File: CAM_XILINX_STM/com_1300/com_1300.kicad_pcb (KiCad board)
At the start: 4 copper layers, 50 x 75.9 mm, 112 parts, among them J1 MEC1-108-01-S-D-RA1-SL, J2 9-68RD-0.635SF, U1 LT1963AxST-3.3, U2 LP3982IMM-ADJ, U3 LTC3411EMS, U5 STM32F415RGTx, U6 AM29LV320DT90EC, U7 TC74LCX373FT, Y1 40mHZ, Y2 16mHz

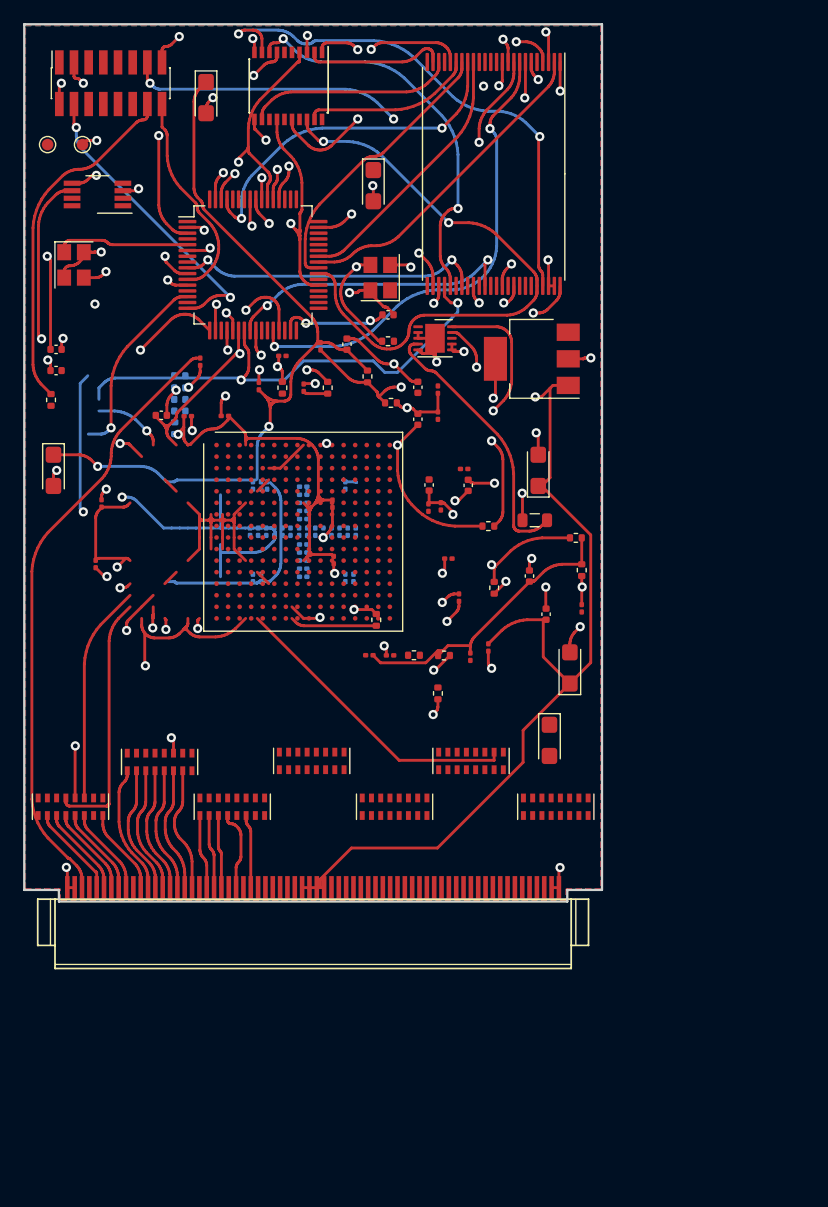
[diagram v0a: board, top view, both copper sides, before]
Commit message: 2342342
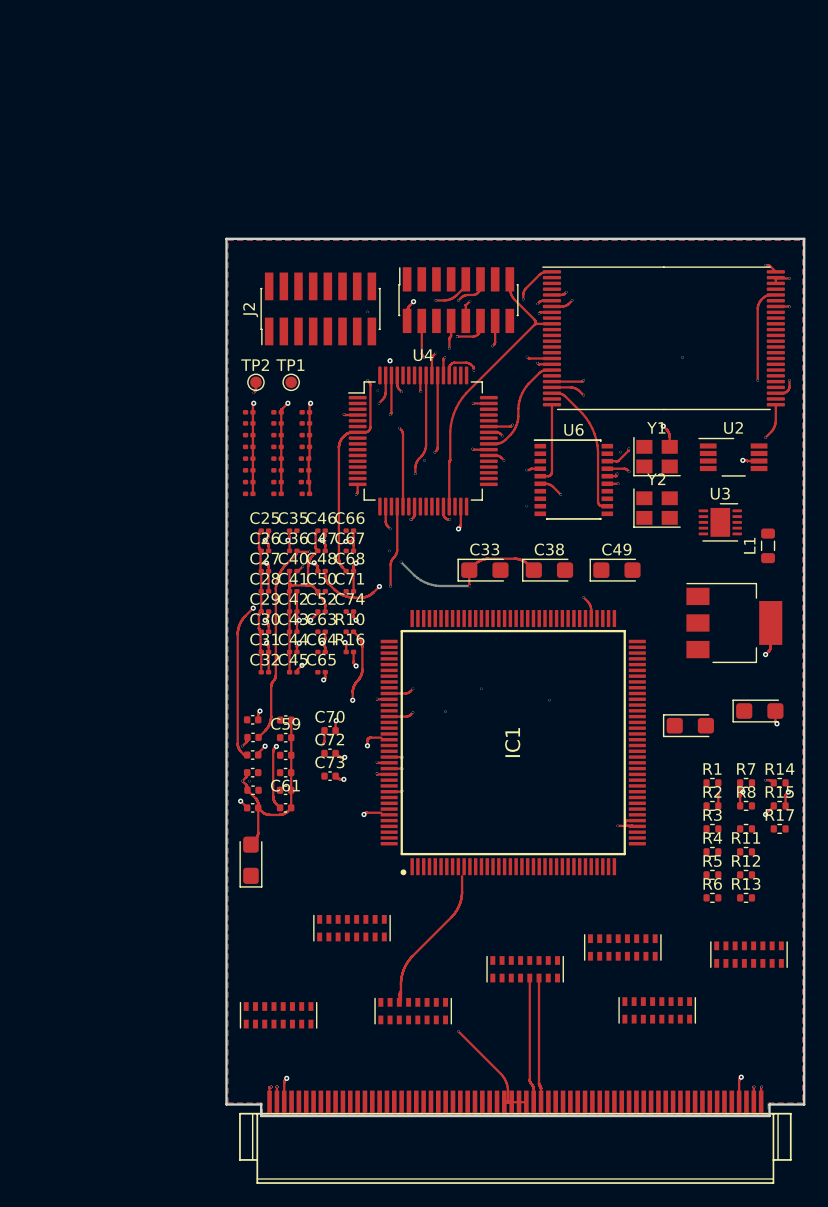
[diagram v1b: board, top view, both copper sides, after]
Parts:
- removed the C24 at (32.4, 39.0)
- removed the C24 at (50.8, 36.7)
- removed the C24 at (50.8, 39.0)
- removed the C24 at (63.2, 55.6)
- removed the C24 at (21.2, 51.8)
- removed the C24 at (17.8, 33.2)
- removed the C24 at (41.7, 46.6)
- removed the C24 at (49.1, 39.3)
- removed the C24 at (21.7, 46.5)
- removed the C24 at (53.6, 59.8)
- removed the C24 at (51.1, 46.8)
- removed the C24 at (50.0, 46.9)
- removed the C24 at (49.1, 36.5)
- removed the C24 at (41.8, 51.4)
- removed the C24 at (17.8, 35.1)
- removed the C24 at (39.1, 46.5)
- removed the C24 at (39.1, 45.8)
- removed the C24 at (36.0, 45.0)
- removed the C24 at (28.5, 37.5)
- removed the C24 at (43.5, 53.0)
- removed the C24 at (39.1, 45.1)
- removed the C24 at (40.2, 49.0)
- removed the C24 at (46.5, 30.2)
- removed the C24 at (43.7, 49.0)
- removed the C24 at (39.1, 47.2)
- removed the C24 at (39.1, 50.8)
- removed the C24 at (43.0, 49.0)
- removed the C24 at (35.2, 49.0)
- removed the C24 at (42.3, 49.0)
- removed the C24 at (35.5, 53.0)
- removed the C24 at (39.1, 52.2)
- removed the C24 at (38.0, 49.0)
- removed the C24 at (34.5, 49.0)
- removed the C24 at (53.4, 45.0)
- removed the C24 at (34.8, 45.0)
- removed the C24 at (39.1, 47.9)
- removed the C24 at (39.1, 52.9)
- removed the C24 at (39.5, 49.0)
- removed the C24 at (40.9, 49.0)
- removed the C24 at (39.1, 51.5)
- removed the C24 at (36.6, 49.0)
- removed the C24 at (42.8, 45.0)
- removed the C24 at (41.6, 49.0)
- removed the C24 at (37.3, 49.0)
- removed the C24 at (29.2, 39.0)
- removed the C24 at (35.9, 49.0)
- removed the C24 at (42.8, 53.0)
- removed the C24 at (34.8, 53.0)
- removed the C24 at (35.5, 45.0)
- removed the C24 at (39.1, 50.1)
- removed the C24 at (38.8, 49.0)
- removed the C24 at (51.7, 51.3)
- removed the C24 at (44.9, 59.7)
- removed the C24 at (53.1, 43.6)
- removed the C24 at (37.3, 33.8)
- removed C39: 10uF, Capacitor_Tantalum_SMD:CP_EIA-3216-18_Kemet-A
- removed C62: C-OPEN, Capacitor_SMD:C_0402_1005Metric
- removed R9: 56, Resistor_SMD:R_0402_1005Metric
- removed U: XC3S400-4FT256C, Package_BGA:Xilinx_FTG256
- removed U7: TC74LCX373FT, Package_SO:SSOP-20_4.4x6.5mm_P0.65mm
- added C24: C-OPEN, Capacitor_SMD:C_0402_1005Metric, F.Cu at (41.5, 66.2)
- added C24: C-OPEN, Capacitor_SMD:C_0201_0603Metric, F.Cu at (38.3, 61.2)
- added C24: C-OPEN, Capacitor_SMD:C_0201_0603Metric, F.Cu at (35.8, 52.4)
- added C24: C-OPEN, Capacitor_SMD:C_0201_0603Metric, F.Cu at (38.3, 54.2)
- added C24: C-OPEN, Capacitor_SMD:C_0201_0603Metric, F.Cu at (39.4, 45.7)
- added C24: C-OPEN, Capacitor_SMD:C_0201_0603Metric, F.Cu at (40.7, 61.2)
- added C24: C-OPEN, Capacitor_SMD:C_0201_0603Metric, F.Cu at (35.8, 57.7)
- added C24: C-OPEN, Capacitor_SMD:C_0402_1005Metric, F.Cu at (37.6, 71.4)
- added C24: C-OPEN, Capacitor_SMD:C_0201_0603Metric, F.Cu at (36.9, 38.7)
- added C24: C-OPEN, Capacitor_SMD:C_0201_0603Metric, F.Cu at (38.3, 52.4)
- added C24: C-OPEN, Capacitor_SMD:C_0201_0603Metric, F.Cu at (35.8, 61.2)
- added C24: C-OPEN, Capacitor_SMD:C_0201_0603Metric, F.Cu at (34.5, 38.7)
- added C24: C-OPEN, Capacitor_SMD:C_0201_0603Metric, F.Cu at (40.7, 50.7)
- added C24: C-OPEN, Capacitor_SMD:C_0201_0603Metric, F.Cu at (43.2, 55.9)
- added C24: C-OPEN, Capacitor_SMD:C_0201_0603Metric, F.Cu at (36.9, 43.7)
- added C24: C-OPEN, Capacitor_SMD:C_0201_0603Metric, F.Cu at (34.5, 40.6)
- added C24: C-OPEN, Capacitor_SMD:C_0201_0603Metric, F.Cu at (36.9, 41.7)
- added C24: C-OPEN, Capacitor_SMD:C_0201_0603Metric, F.Cu at (40.7, 57.7)
- added C24: C-OPEN, Capacitor_SMD:C_0201_0603Metric, F.Cu at (38.3, 57.7)
- added C24: C-OPEN, Capacitor_SMD:C_0201_0603Metric, F.Cu at (38.3, 59.4)
- added C24: C-OPEN, Capacitor_SMD:C_0201_0603Metric, F.Cu at (34.5, 39.6)
- added C24: C-OPEN, Capacitor_SMD:C_0201_0603Metric, F.Cu at (36.9, 42.7)
- added C24: C-OPEN, Capacitor_SMD:C_0201_0603Metric, F.Cu at (34.5, 43.7)
- added C24: C-OPEN, Capacitor_SMD:C_0402_1005Metric, F.Cu at (34.8, 68.3)
- added C24: C-OPEN, Capacitor_SMD:C_0201_0603Metric, F.Cu at (39.3, 42.7)
- added C24: C-OPEN, Capacitor_SMD:C_0201_0603Metric, F.Cu at (35.8, 55.9)
- added C24: C-OPEN, Capacitor_SMD:C_0201_0603Metric, F.Cu at (35.8, 54.2)
- added C24: C-OPEN, Capacitor_SMD:C_0201_0603Metric, F.Cu at (34.5, 41.7)
- added C24: C-OPEN, Capacitor_SMD:C_0201_0603Metric, F.Cu at (36.9, 39.6)
- added C24: C-OPEN, Capacitor_SMD:C_0201_0603Metric, F.Cu at (39.3, 43.7)
- added C24: C-OPEN, Capacitor_SMD:C_0201_0603Metric, F.Cu at (35.8, 59.4)
- added C24: C-OPEN, Capacitor_SMD:C_0201_0603Metric, F.Cu at (36.9, 44.7)
- added C24: C-OPEN, Capacitor_SMD:C_0201_0603Metric, F.Cu at (34.5, 42.7)
- added C24: C-OPEN, Capacitor_SMD:C_0201_0603Metric, F.Cu at (35.8, 50.7)
- added C24: C-OPEN, Capacitor_SMD:C_0402_1005Metric, F.Cu at (37.6, 72.9)
- added C24: C-OPEN, Capacitor_SMD:C_0201_0603Metric, F.Cu at (34.5, 44.7)
- added C24: C-OPEN, Capacitor_SMD:C_0201_0603Metric, F.Cu at (43.2, 54.2)
- added C24: C-OPEN, Capacitor_SMD:C_0201_0603Metric, F.Cu at (43.2, 52.4)
- added C24: C-OPEN, Capacitor_SMD:C_0201_0603Metric, F.Cu at (36.9, 45.7)
- added C24: C-OPEN, Capacitor_SMD:C_0201_0603Metric, F.Cu at (40.7, 48.9)
- added C24: C-OPEN, Capacitor_SMD:C_0402_1005Metric, F.Cu at (41.5, 68.2)
- added C24: C-OPEN, Capacitor_SMD:C_0201_0603Metric, F.Cu at (36.9, 40.6)
- added C24: C-OPEN, Capacitor_SMD:C_0402_1005Metric, F.Cu at (34.8, 65.3)
- added C24: C-OPEN, Capacitor_SMD:C_0201_0603Metric, F.Cu at (39.4, 38.7)
- added C24: C-OPEN, Capacitor_SMD:C_0201_0603Metric, F.Cu at (35.8, 48.9)
- added C24: C-OPEN, Capacitor_SMD:C_0201_0603Metric, F.Cu at (40.7, 59.4)
- added C24: C-OPEN, Capacitor_SMD:C_0201_0603Metric, F.Cu at (39.4, 41.7)
- added C24: C-OPEN, Capacitor_SMD:C_0201_0603Metric, F.Cu at (34.5, 45.7)
- added C24: C-OPEN, Capacitor_SMD:C_0201_0603Metric, F.Cu at (43.2, 50.7)
- added C24: C-OPEN, Capacitor_SMD:C_0201_0603Metric, F.Cu at (39.3, 44.7)
- added C24: C-OPEN, Capacitor_SMD:C_0201_0603Metric, F.Cu at (43.2, 48.9)
- added C24: C-OPEN, Capacitor_SMD:C_0201_0603Metric, F.Cu at (38.3, 55.9)
- added C24: C-OPEN, Capacitor_SMD:C_0201_0603Metric, F.Cu at (39.4, 39.6)
- added C24: C-OPEN, Capacitor_SMD:C_0402_1005Metric, F.Cu at (41.5, 70.2)
- added C24: C-OPEN, Capacitor_SMD:C_0201_0603Metric, F.Cu at (39.4, 40.6)
- added C38: 10uF, Capacitor_Tantalum_SMD:CP_EIA-3216-18_Kemet-A, F.Cu at (60.5, 52.3)
- added C48: 100nF, Capacitor_SMD:C_0201_0603Metric, F.Cu at (40.7, 52.4)
- added IC1: XC3S400-4TQ144C, SUNfWGlsaW54X1hDM1MyMDAtNFRRRzE0NEMuemlw:QFP50P2200X2200X160-144N, F.Cu at (57.3, 67.2)
- added J2: Conn_02x10_Top_Bottom, Connector_PinHeader_1.27mm:PinHeader_2x08_P1.27mm_Vertical_SMD, F.Cu at (40.6, 29.7)
- added R8: R-OPEN, Resistor_SMD:R_0402_1005Metric, F.Cu at (77.5, 72.7)
- added U4: STM32F415RGTx, Package_QFP:LQFP-64_10x10mm_P0.5mm, F.Cu at (49.5, 41.1)
- C49: value C-OPEN -> 10uF; footprint Capacitor_SMD:C_0402_1005Metric -> Capacitor_Tantalum_SMD:CP_EIA-3216-18_Kemet-A
- C50: value C-OPEN -> 22pF; footprint Capacitor_SMD:C_0402_1005Metric -> Capacitor_SMD:C_0201_0603Metric; moved to F.Cu
- C51: value C-OPEN -> 10uF; footprint Capacitor_SMD:C_0402_1005Metric -> Capacitor_Tantalum_SMD:CP_EIA-3216-18_Kemet-A; moved to F.Cu
- C53: value 10uF -> 4.7uF; footprint Capacitor_Tantalum_SMD:CP_EIA-3216-18_Kemet-A -> Capacitor_SMD:C_0402_1005Metric
- C54: value 22pF -> 10uF; footprint Capacitor_SMD:C_0201_0603Metric -> Capacitor_Tantalum_SMD:CP_EIA-3216-18_Kemet-A
- C56: value 100nF -> 4.7uF; footprint Capacitor_SMD:C_0201_0603Metric -> Capacitor_SMD:C_0402_1005Metric
- C57, C60: value 4.7uF -> C-OPEN
- C58, C59: value 10uF -> C-OPEN; footprint Capacitor_Tantalum_SMD:CP_EIA-3216-18_Kemet-A -> Capacitor_SMD:C_0402_1005Metric
- C61, R22: moved to F.Cu
- R10: value 100K -> 0; footprint Resistor_SMD:R_0402_1005Metric -> Resistor_SMD:R_0201_0603Metric
- R11: value 100K -> 4.7K
- R12: value R-OPEN -> 330
- R13: value 0 -> 56; footprint Resistor_SMD:R_0201_0603Metric -> Resistor_SMD:R_0402_1005Metric
- R4: value 330 -> 100K
- R5: value 4.7K -> 49.9K
- R7: value 49.9K -> 100K
- U5: value STM32F415RGTx -> AM29LV320DT90EC; footprint Package_QFP:LQFP-64_10x10mm_P0.5mm -> Package_SO:TSOP-I-48_18.4x12mm_P0.5mm
- U6: value AM29LV320DT90EC -> TC74LCX373FT; footprint Package_SO:TSOP-I-48_18.4x12mm_P0.5mm -> Package_SO:SSOP-20_4.4x6.5mm_P0.65mm
- moved R14 71.2 mm to (80.4, 70.7), turned to 0 degrees
- moved R22 60.4 mm to (77.5, 74.7), turned to 0 degrees
- moved U2 59.6 mm to (76.4, 42.6), turned to 0 degrees
- moved Y2 54.7 mm to (69.8, 47.0), turned to 0 degrees
- moved C58 54.3 mm to (37.6, 65.3), turned to 180 degrees
- moved R3 53.3 mm to (74.6, 74.7), turned to 0 degrees
- moved C53 51.9 mm to (34.8, 69.8), turned to 0 degrees
- moved R6 51.1 mm to (74.6, 80.7), turned to 0 degrees
- moved C54 49.4 mm to (78.7, 64.5), turned to 0 degrees
- moved R2 49.0 mm to (74.6, 72.7), turned to 0 degrees
- moved R7 48.1 mm to (77.5, 70.7), turned to 0 degrees
- moved R1 47.7 mm to (74.6, 70.7), turned to 0 degrees
- moved C49 41.6 mm to (66.3, 52.3), turned to 0 degrees
- moved C51 41.3 mm to (34.6, 77.4), turned to 90 degrees
- moved R13 37.3 mm to (77.5, 80.7), turned to 0 degrees
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- renumbered J2 to J3
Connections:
- C49 pad 1: GND -> +3V3
- C49 pad 2: uC_CNTRL1 -> GND
- C50 pad 1: GND -> +1V2
- C50 pad 2: uC_CNTRL4 -> Net-(U3-VFB)
- C51 pad 1: GND -> +3V3
- C51 pad 2: uC_CNTRL2 -> GND
- C52 pad 2: Net-(U2-CC) -> +1V2
- C53 pad 1: +3V3 -> GND
- C53 pad 2: GND -> +2V5
- C54 pad 2: Net-(U3-VFB) -> GND
- C55 pad 1: +3V3 -> +1V2
- C57 pad 1: GND -> /FPGA_CLK1
- C57 pad 2: +2V5 -> GND
- C58 pad 1: +1V2 -> GND
- C58 pad 2: GND -> uC_CNTRL1
- C59 pad 1: +1V2 -> 40MHz_OSC
- C60 pad 2: +1V2 -> uC_CNTRL2
- C61 pad 1: /FPGA_CLK1 -> GND
- C61 pad 2: GND -> uC_CNTRL4
- R10 pad 1: Net-(U2-SET) -> Net-(IC1-IO_L32P_4/GCLK0)
- R10 pad 2: +2V5 -> /FPGA_CLK1
- R11 pad 1: GND -> +3V3
- R11 pad 2: Net-(U2-SET) -> Net-(IC1-IO_L31N_4/INIT_B)
- R12 pad 1: GND -> +2V5
- R12 pad 2: +2V5 -> FPGA_CNTRL3
- R13 pad 1: Net-(U4-IO_L32N_4/GCLK1) -> uC_CNTRL2
- R13 pad 2: /FPGA_CLK1 -> Net-(IC1-CCLK)
- R4 pad 1: +2V5 -> GND
- R4 pad 2: FPGA_CNTRL3 -> Net-(U3-VFB)
- R5 pad 1: +3V3 -> +1V2
- R5 pad 2: Net-(U4-IO_L31N_4/INIT_B) -> Net-(U3-VFB)
- R6 pad 1: GND -> Net-(U2-SET)
- R6 pad 2: Net-(U3-VFB) -> +2V5
- R7 pad 1: +1V2 -> GND
- R7 pad 2: Net-(U3-VFB) -> Net-(U2-SET)
- RN2 pad 1: unconnected-(RN2-R1.1-Pad1) -> INOUT_MCLKO
- RN2 pad 16: unconnected-(RN2-R1.2-Pad16) -> MCLKO
- RN4 pad 2: INOUT_D2 -> INOUT_D4
- RN7 pad 13: MCLKO -> unconnected-(RN7-R4.2-Pad13)
- RN7 pad 4: INOUT_MCLKO -> unconnected-(RN7-R4.1-Pad4)
- TP1 pad 1: FPGA_CNTRL3 -> Net-(IC1-IO_L31N_4/INIT_B)
- TP2 pad 1: Net-(U4-IO_L31N_4/INIT_B) -> FPGA_CNTRL3
- U5 pad 1: +3V3 -> uC_A16
- U5 pad 10: uC_PROG1 -> uC_PROG2
- U5 pad 11: uC_PROG4 -> uC_CNTRL1
- U5 pad 12: GND -> +3V3
- U5 pad 13: +3V3 -> unconnected-(U5-NC-Pad13)
- U5 pad 14: FPGA_CNTRL1 -> +3V3
- U5 pad 16: SERIAL_TX -> uC_A19
- U5 pad 17: SERIAL_RX -> uC_A18
- U5 pad 18: GND -> uC_A8
- U5 pad 19: +3V3 -> uC_A7
- U5 pad 2: uC_A14 -> uC_A15
- U5 pad 20: FPGA_CNTRL2 -> uC_A6
- U5 pad 21: FPGA_CNTRL3 -> uC_A5
- U5 pad 22: uC_CNTRL1 -> uC_A4
- U5 pad 23: uC_CNTRL2 -> uC_A3
- U5 pad 24: uC_AD3 -> uC_A2
- U5 pad 25: uC_AD4 -> uC_A1
- U5 pad 26: unconnected-(U5-PB0-Pad26) -> uC_CNTRL3
- U5 pad 27: unconnected-(U5-PB1-Pad27) -> GND
- U5 pad 28: uC_A9 -> uC_CNTRL2
- U5 pad 29: uC_PROG2 -> uC_AD0
- U5 pad 3: uC_A13 -> uC_A14
- U5 pad 31: Net-(U5-VCAP_1) -> uC_AD1
- U5 pad 32: +3V3 -> unconnected-(U5-DQ9-Pad32)
- U5 pad 33: unconnected-(U5-PB12-Pad33) -> uC_AD2
- U5 pad 35: unconnected-(U5-PB14-Pad35) -> uC_AD3
- U5 pad 37: uC_AD5 -> +3V3
- U5 pad 38: uC_AD6 -> uC_AD4
- U5 pad 39: uC_AD7 -> unconnected-(U5-DQ12-Pad39)
- U5 pad 4: uC_A12 -> uC_A13
- U5 pad 40: uC_A8 -> uC_AD5
- U5 pad 41: uC_A15 -> unconnected-(U5-DQ13-Pad41)
- U5 pad 42: uC_A19 -> uC_AD6
- U5 pad 43: INOUT_PC_CARD_55 -> unconnected-(U5-DQ14-Pad43)
- U5 pad 44: unconnected-(U5-PA11-Pad44) -> uC_AD7
- U5 pad 45: unconnected-(U5-PA12-Pad45) -> uC_A0
- U5 pad 46: unconnected-(U5-PA13-Pad46) -> GND
- U5 pad 47: Net-(U5-VCAP_2) -> GND
- U5 pad 48: +3V3 -> uC_A17
- U5 pad 5: OSC_IN -> uC_A12
- U5 pad 6: OSC_OUT -> uC_A11
- U5 pad 7: NRST -> uC_A10
- U5 pad 8: uC_AD0 -> uC_A9
- U5 pad 9: uC_AD1 -> uC_PROG1
- U6 pad 1: uC_A16 -> GND
- U6 pad 10: uC_PROG2 -> GND
- U6 pad 11: uC_CNTRL1 -> uC_CNTRL4
- U6 pad 12: +3V3 -> uC_A4
- U6 pad 13: unconnected-(U6-NC-Pad13) -> uC_AD4
- U6 pad 14: +3V3 -> uC_AD5
- U6 pad 15: unconnected-(U6-RY/BY#-Pad15) -> uC_A5
- U6 pad 16: uC_A19 -> uC_A6
- U6 pad 17: uC_A18 -> uC_AD6
- U6 pad 18: uC_A8 -> uC_AD7
- U6 pad 2: uC_A15 -> uC_A3
- U6 pad 20: uC_A6 -> +3V3
- U6 pad 3: uC_A14 -> uC_AD3
- U6 pad 4: uC_A13 -> uC_AD2
- U6 pad 5: uC_A12 -> uC_A2
- U6 pad 6: uC_A11 -> uC_A1
- U6 pad 7: uC_A10 -> uC_AD1
- U6 pad 8: uC_A9 -> uC_AD0
- U6 pad 9: uC_PROG1 -> uC_A0
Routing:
- net +2V5: track 120.1 -> 12.5 mm, vias 3 -> 0
- net +1V2: track 122.0 -> 21.7 mm, vias 3 -> 0
- net uC_AD4: track 80.5 -> 0.00 mm, vias 3 -> 0
- net Net-(U2-SET): track 71.0 -> 0.00 mm, vias 2 -> 0
- net uC_A14: track 66.8 -> 0.00 mm, vias 2 -> 0
- net uC_PROG1: track 58.4 -> 0.00 mm, vias 4 -> 0
- net NRST: track 30.6 -> 87.5 mm, vias 0 -> 4
- net uC_AD3: track 51.7 -> 0.00 mm, vias 3 -> 0
- net uC_CNTRL1: track 51.5 -> 0.00 mm, vias 2 -> 0
- net uC_CNTRL2: track 69.4 -> 20.4 mm, vias 3 -> 2
- net FPGA_CNTRL3: track 70.4 -> 21.5 mm, vias 5 -> 2
- net FPGA_TEST_EDGE3: track 0.00 -> 48.4 mm, vias 0 -> 2
- net uC_AD2: track 64.8 -> 16.5 mm, vias 3 -> 2
- net Net-(C73-Pad1): track 47.9 -> 0.00 mm, vias 2 -> 0
- net uC_A13: track 47.3 -> 0.00 mm, vias 2 -> 0
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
